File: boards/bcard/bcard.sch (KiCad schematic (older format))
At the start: 13 parts, among them IC1 ATTINY10-TS, P1 BATT, Q1 BC846A

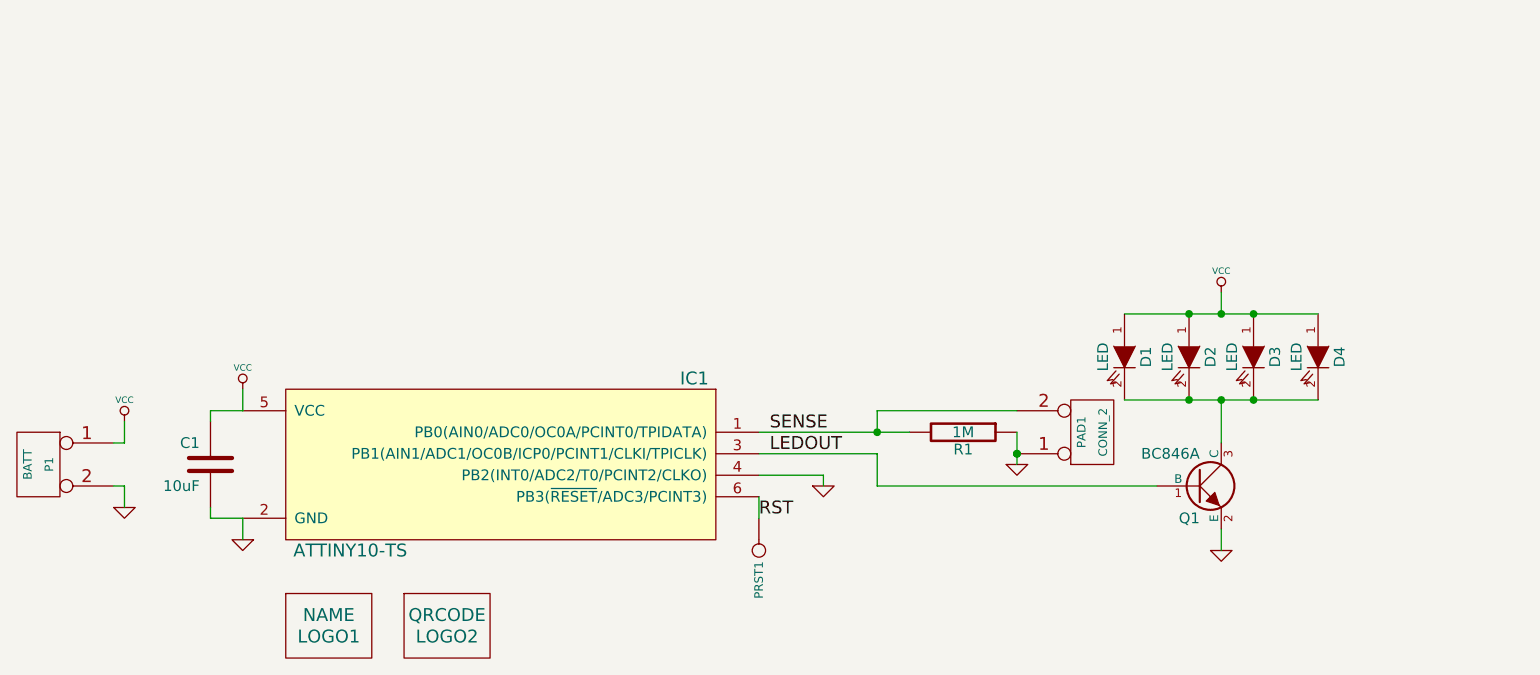
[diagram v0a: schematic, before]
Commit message: first pcb design basically done
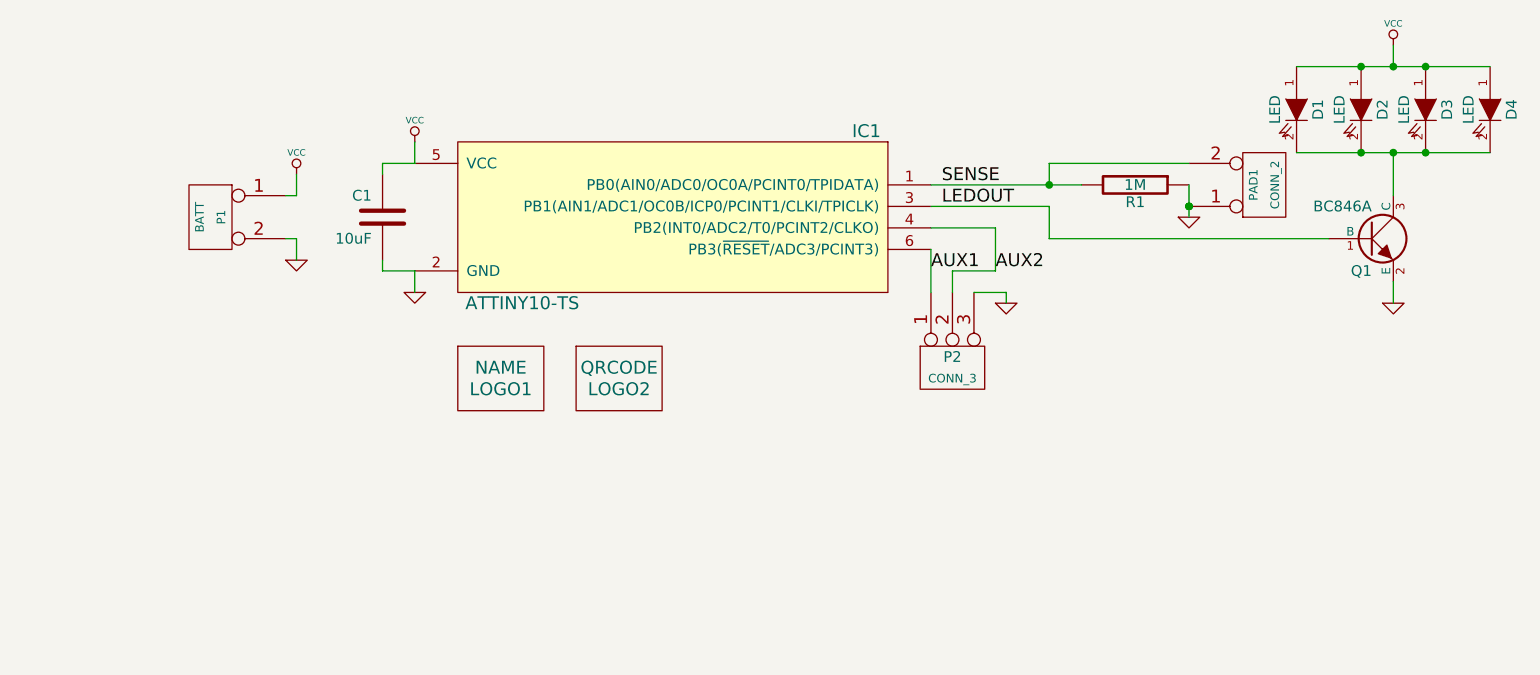
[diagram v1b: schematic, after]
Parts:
- removed PRST1: CONN_1, symbol CONN_1
- added P2: CONN_3, symbol CONN_3
- D1, D2, D3, D4: footprint LED-1206-3D -> SM1206POL
- IC1: footprint DIP-28__300 -> SOT23_6
- LOGO1: footprint (none) -> LOGO
- LOGO2: footprint (none) -> JWCXZ
- PAD1: footprint (none) -> CAPSENSE
- R1: footprint SM0805 -> SM0603
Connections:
- net GND: now also P2.3 (P3); no longer IC1.4 (PB2(INT0/ADC2/T0/PCINT2/CLKO))
- net RST renamed AUX1
- net AUX1: now also P2.1 (P1)
- new net AUX2: IC1.4 (PB2(INT0/ADC2/T0/PCINT2/CLKO)), P2.2 (PM)
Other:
- moved on the sheet: C1, D1, D2, D3, D4, IC1, LOGO1, LOGO2, P1, PAD1, Q1, R1

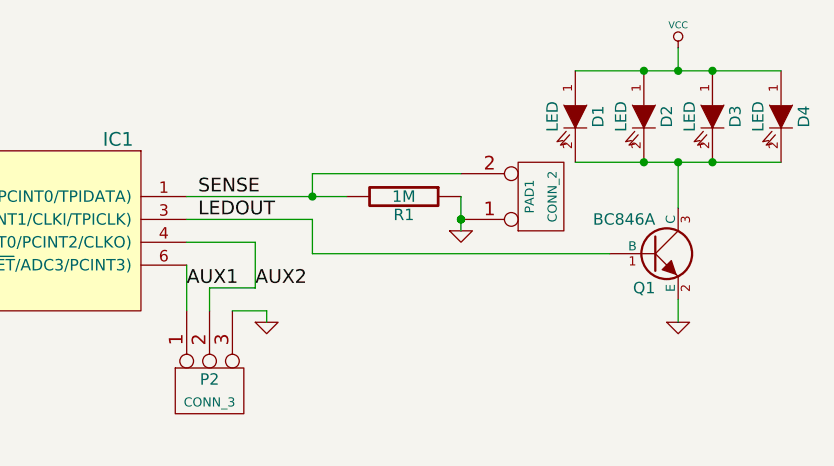
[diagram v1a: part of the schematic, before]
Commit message: almost done with new style
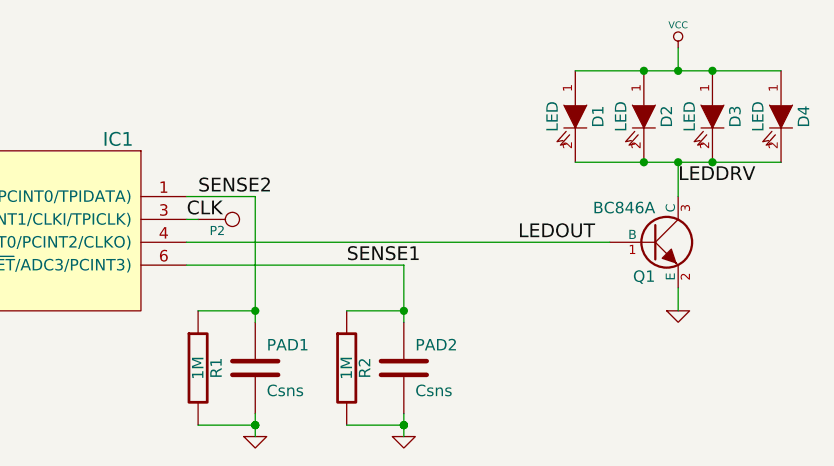
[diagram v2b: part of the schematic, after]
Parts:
- removed P2: CONN_3, symbol CONN_3
- removed PAD1: CONN_2, CAPSENSE, symbol CONN_2
- added P2: CONN_1, PAD, symbol CONN_1
- added PAD1, PAD2: Csns, SIL-2, symbol C
- added R2: 1M, SM0603, symbol R
- D1, D2, D3, D4: footprint SM1206POL -> LED-3mmS
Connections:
- net AUX2 is gone; now on net LEDOUT: IC1.4 (PB2(INT0/ADC2/T0/PCINT2/CLKO))
- net GND: now also R1.2, PAD1.2, PAD2.2, R2.2; no longer R1.1
- net LEDOUT: no longer IC1.3 (PB1(AIN1/ADC1/OC0B/ICP0/PCINT1/CLKI/TPICLK))
- net LEDDRV: now reaches D1.2 (K), D2.2 (K), D3.2 (K), D4.2 (K), Q1.3 (C)
- net AUX1 renamed SENSE1
- net SENSE1: now also PAD2.1, R2.1
- net SENSE renamed SENSE2
- net SENSE2: now also R1.1, PAD1.1; no longer R1.2
- new net CLK: IC1.3 (PB1(AIN1/ADC1/OC0B/ICP0/PCINT1/CLKI/TPICLK)), P2.1
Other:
- moved on the sheet: Q1, R1
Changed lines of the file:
@@
-EESchema Schematic File Version 2  date Thu 29 Mar 2012 05:30:36 PM EDT
+EESchema Schematic File Version 2  date Fri 25 May 2012 11:36:53 AM EDT
 LIBS:power
 LIBS:device
@@
 Sheet 1 1
 Title "bcard"
-Date "29 mar 2012"
+Date "25 may 2012"
 Rev "1.0"
 Comp "J. Colosimo"
@@
 F 0 "D4" H 8600 3150 50  0000 C CNN
 F 1 "LED" H 8600 2950 50  0000 C CNN
-F 2 "SM1206POL" H 8600 3050 50  0001 C CNN
+F 2 "LED-3mmS" H 8600 3050 50  0001 C CNN
 F 4 "APT3216QBC/D" H 8600 3050 60  0001 C CNN "Part"
 F 5 "http://search.digikey.com/us/en/products/APT3216QBC%2FD/754-1439-1-ND/2163797" H 8600 3050 60  0001 C CNN "URL"
@@
 F 0 "D3" H 8300 3150 50  0000 C CNN
 F 1 "LED" H 8300 2950 50  0000 C CNN
-F 2 "SM1206POL" H 8300 3050 50  0001 C CNN
+F 2 "LED-3mmS" H 8300 3050 50  0001 C CNN
 F 4 "APT3216QBC/D" H 8300 3050 60  0001 C CNN "Part"
 F 5 "http://search.digikey.com/us/en/products/APT3216QBC%2FD/754-1439-1-ND/2163797" H 8300 3050 60  0001 C CNN "URL"
@@
 F 0 "D2" H 8000 3150 50  0000 C CNN
 F 1 "LED" H 8000 2950 50  0000 C CNN
-F 2 "SM1206POL" H 8000 3050 50  0001 C CNN
+F 2 "LED-3mmS" H 8000 3050 50  0001 C CNN
 F 4 "APT3216QBC/D" H 8000 3050 60  0001 C CNN "Part"
 F 5 "http://search.digikey.com/us/en/products/APT3216QBC%2FD/754-1439-1-ND/2163797" H 8000 3050 60  0001 C CNN "URL"
@@
 L R R1
 U 1 1 4F57ACF5
-P 6950 3400
-F 0 "R1" V 7030 3400 50  0000 C CNN
-F 1 "1M" V 6950 3400 50  0000 C CNN
-F 2 "SM0603" V 7050 3400 50  0001 C CNN
-F 4 "RC0603JR-071ML" V 6950 3400 60  0001 C CNN "Part"
-F 5 "http://search.digikey.com/us/en/products/RC0603JR-071ML/311-1.0MGRCT-ND/729625" V 6950 3400 60  0001 C CNN "URL"
-	1    6950 3400
-	0    1    1    0
+P 6050 4150
+F 0 "R1" V 6130 4150 50  0000 C CNN
+F 1 "1M" V 6050 4150 50  0000 C CNN
+F 2 "SM0603" V 6150 4150 50  0001 C CNN
+F 4 "RC0603JR-071ML" V 6050 4150 60  0001 C CNN "Part"
+F 5 "http://search.digikey.com/us/en/products/RC0603JR-071ML/311-1.0MGRCT-ND/729625" V 6050 4150 60  0001 C CNN "URL"
+	1    6050 4150
+	1    0    0    -1
 $EndComp
 $Comp
@@
 L GND #PWR03
 U 1 1 4F57A9AD
-P 8150 3950
-F 0 "#PWR03" H 8150 3950 30  0001 C CNN
-F 1 "GND" H 8150 3880 30  0001 C CNN
-	1    8150 3950
+P 8150 3900
+F 0 "#PWR03" H 8150 3900 30  0001 C CNN
+F 1 "GND" H 8150 3830 30  0001 C CNN
+	1    8150 3900
 	1    0    0    -1
 $EndComp
@@
 F 0 "D1" H 7700 3150 50  0000 C CNN
 F 1 "LED" H 7700 2950 50  0000 C CNN
-F 2 "SM1206POL" H 7700 3050 50  0001 C CNN
+F 2 "LED-3mmS" H 7700 3050 50  0001 C CNN
 F 4 "APT3216QBC/D" H 7700 3050 60  0001 C CNN "Part"
 F 5 "http://search.digikey.com/us/en/products/APT3216QBC%2FD/754-1439-1-ND/2163797" H 7700 3050 60  0001 C CNN "URL"
@@
 L BC846A Q1
 U 1 1 4F57A871
-P 8050 3650
-F 0 "Q1" H 8050 3500 50  0000 R CNN
-F 1 "BC846A" H 8050 3800 50  0000 R CNN
-F 2 "SOT323" H 8050 3900 50  0001 C CNN
-F 4 "BC846A" H 8050 3650 60  0001 C CNN "Part"
-F 5 "http://search.digikey.com/us/en/products/BC846A,215/568-4866-1-ND/2122195" H 8050 3650 60  0001 C CNN "URL"
-	1    8050 3650
+P 8050 3600
+F 0 "Q1" H 8050 3450 50  0000 R CNN
+F 1 "BC846A" H 8050 3750 50  0000 R CNN
+F 2 "SOT323" H 8050 3850 50  0001 C CNN
+F 4 "BC846A" H 8050 3600 60  0001 C CNN "Part"
+F 5 "http://search.digikey.com/us/en/products/BC846A,215/568-4866-1-ND/2122195" H 8050 3600 60  0001 C CNN "URL"
+	1    8050 3600
 	1    0    0    -1
 $EndComp
@@
 $EndComp
 $Comp
-L GND #PWR07
-U 1 1 4F72D7B3
-P 7200 3550
-F 0 "#PWR07" H 7200 3550 30  0001 C CNN
-F 1 "GND" H 7200 3480 30  0001 C CNN
-	1    7200 3550
-	1    0    0    -1
-$EndComp
-$Comp
 L LOGO LOGO1
 U 1 1 4F737976
@@
 	1    0    0    -1
 $EndComp
+Text Label 6050 3400 0    60   ~ 0
+SENSE2
+Text Label 7450 3600 0    60   ~ 0
+LEDOUT
 $Comp
 L LOGO LOGO2
@@
 	1    0    0    -1
 $EndComp
-Text Label 6050 3400 0    60   ~ 0
-SENSE
-Text Label 6050 3500 0    60   ~ 0
-LEDOUT
-Text Label 6000 3800 0    60   ~ 0
-AUX1
-$Comp
-L CONN_2 PAD1
-U 1 1 4F740194
-P 7550 3400
-F 0 "PAD1" V 7500 3400 40  0000 C CNN
-F 1 "CONN_2" V 7600 3400 40  0000 C CNN
-F 2 "CAPSENSE" V 7700 3400 40  0001 C CNN
-	1    7550 3400
-	1    0    0    1
-$EndComp
-Text Label 6300 3800 0    60   ~ 0
-AUX2
-$Comp
-L CONN_3 P2
-U 1 1 4F74D36B
-P 6100 4250
-F 0 "P2" V 6050 4250 50  0000 C CNN
-F 1 "CONN_3" V 6150 4250 40  0000 C CNN
-	1    6100 4250
-	0    -1   1    0
+Text Label 8150 3350 0    60   ~ 0
+LEDDRV
+$Comp
+L C PAD1
+U 1 1 4FBF9DE9
+P 6300 4150
+F 0 "PAD1" H 6350 4250 50  0000 L CNN
+F 1 "Csns" H 6350 4050 50  0000 L CNN
+F 2 "SIL-2" H 6350 4150 50  0001 C CNN
+	1    6300 4150
+	1    0    0    -1
+$EndComp
+$Comp
+L GND #PWR07
+U 1 1 4FBF9E84
+P 6300 4450
+F 0 "#PWR07" H 6300 4450 30  0001 C CNN
+F 1 "GND" H 6300 4380 30  0001 C CNN
+	1    6300 4450
+	1    0    0    -1
+$EndComp
+$Comp
+L R R2
+U 1 1 4FBF9F06
+P 6700 4150
+F 0 "R2" V 6780 4150 50  0000 C CNN
+F 1 "1M" V 6700 4150 50  0000 C CNN
+F 2 "SM0603" V 6800 4150 50  0001 C CNN
+F 4 "RC0603JR-071ML" V 6700 4150 60  0001 C CNN "Part"
+F 5 "http://search.digikey.com/us/en/products/RC0603JR-071ML/311-1.0MGRCT-ND/729625" V 6700 4150 60  0001 C CNN "URL"
+	1    6700 4150
+	1    0    0    -1
+$EndComp
+$Comp
+L C PAD2
+U 1 1 4FBF9F0C
+P 6950 4150
+F 0 "PAD2" H 7000 4250 50  0000 L CNN
+F 1 "Csns" H 7000 4050 50  0000 L CNN
+F 2 "SIL-2" H 7000 4150 50  0001 C CNN
+	1    6950 4150
+	1    0    0    -1
 $EndComp
 $Comp
 L GND #PWR08
-U 1 1 4F74D45B
-P 6350 3950
-F 0 "#PWR08" H 6350 3950 30  0001 C CNN
-F 1 "GND" H 6350 3880 30  0001 C CNN
-	1    6350 3950
+U 1 1 4FBF9F12
+P 6950 4450
+F 0 "#PWR08" H 6950 4450 30  0001 C CNN
+F 1 "GND" H 6950 4380 30  0001 C CNN
+	1    6950 4450
+	1    0    0    -1
+$EndComp
+Text Label 6700 3700 0    60   ~ 0
+SENSE1
+$Comp
+L CONN_1 P2
+U 1 1 4FBFA0FD
+P 6200 3500
+F 0 "P2" H 6100 3450 40  0000 L CNN
+F 1 "CONN_1" H 6200 3555 30  0001 C CNN
+F 2 "PAD" H 6200 3655 30  0001 C CNN
+	1    6200 3500
 	1    0    0    -1
 $EndComp
@@
 Connection ~ 8300 2850
 Wire Wire Line
-	8150 3250 8150 3450
+	8150 3250 8150 3400
 Connection ~ 8150 3250
 Wire Wire Line
-	8150 3850 8150 3950
+	8150 3800 8150 3900
 Wire Wire Line
 	3000 3650 3050 3650
@@
 	3050 3650 3050 3750
 Wire Wire Line
-	6000 3400 6700 3400
-Wire Wire Line
-	7200 3300 6550 3300
-Wire Wire Line
-	6550 3300 6550 3400
-Connection ~ 6550 3400
-Wire Wire Line
-	6000 3500 6550 3500
-Wire Wire Line
-	6550 3500 6550 3650
-Wire Wire Line
-	6550 3650 7850 3650
-Wire Wire Line
-	7200 3550 7200 3400
-Connection ~ 7200 3500
-Connection ~ 7200 3500
-Wire Wire Line
-	6000 3700 6000 3900
-Wire Wire Line
-	6000 3600 6300 3600
-Wire Wire Line
-	6300 3600 6300 3800
-Wire Wire Line
-	6300 3800 6100 3800
-Wire Wire Line
-	6100 3800 6100 3900
-Wire Wire Line
-	6350 3950 6350 3900
-Wire Wire Line
-	6350 3900 6200 3900
+	6000 3600 7850 3600
+Wire Wire Line
+	6050 3900 6300 3900
+Wire Wire Line
+	6300 3950 6300 3400
+Wire Wire Line
+	6300 4350 6300 4450
+Wire Wire Line
+	6300 4400 6050 4400
+Connection ~ 6300 4400
+Connection ~ 6300 4400
+Wire Wire Line
+	6700 3900 6950 3900
+Wire Wire Line
+	6950 3950 6950 3700
+Wire Wire Line
+	6950 4350 6950 4450
+Wire Wire Line
+	6950 4400 6700 4400
+Connection ~ 6950 4400
+Connection ~ 6950 4400
+Wire Wire Line
+	6300 3400 6000 3400
+Connection ~ 6300 3900
+Wire Wire Line
+	6950 3700 6000 3700
+Connection ~ 6950 3900
+Wire Wire Line
+	6000 3500 6050 3500
+Text Label 6000 3500 0    60   ~ 0
+CLK
 $EndSCHEMATC

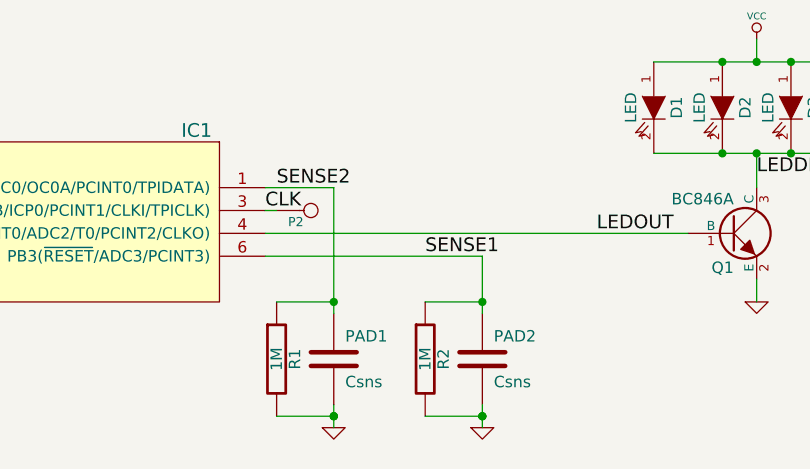
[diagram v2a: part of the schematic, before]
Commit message: finished next revision of bcard -- ready to etch
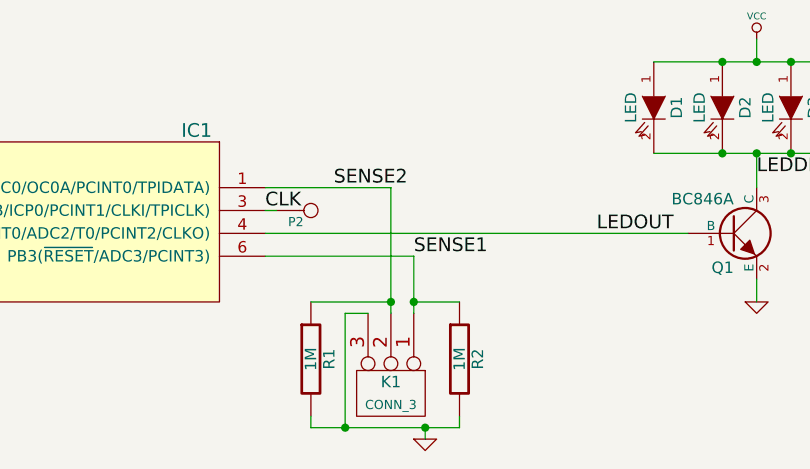
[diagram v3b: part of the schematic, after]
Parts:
- removed PAD1, PAD2: Csns, SIL-2, symbol C
- added K1: CONN_3, SENSOR2, symbol CONN_3
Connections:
- net GND: now also K1.3 (P3)
- net SENSE1: now also K1.1 (P1)
- net SENSE2: now also K1.2 (PM)
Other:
- moved on the sheet: R1, R2
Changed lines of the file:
@@
-EESchema Schematic File Version 2  date Fri 25 May 2012 11:36:53 AM EDT
+EESchema Schematic File Version 2  date Mon 28 May 2012 02:41:33 PM EDT
 LIBS:power
 LIBS:device
@@
 Sheet 1 1
 Title "bcard"
-Date "25 may 2012"
+Date "28 may 2012"
 Rev "1.0"
 Comp "J. Colosimo"
@@
 L R R1
 U 1 1 4F57ACF5
-P 6050 4150
-F 0 "R1" V 6130 4150 50  0000 C CNN
-F 1 "1M" V 6050 4150 50  0000 C CNN
-F 2 "SM0603" V 6150 4150 50  0001 C CNN
-F 4 "RC0603JR-071ML" V 6050 4150 60  0001 C CNN "Part"
-F 5 "http://search.digikey.com/us/en/products/RC0603JR-071ML/311-1.0MGRCT-ND/729625" V 6050 4150 60  0001 C CNN "URL"
-	1    6050 4150
+P 6200 4150
+F 0 "R1" V 6280 4150 50  0000 C CNN
+F 1 "1M" V 6200 4150 50  0000 C CNN
+F 2 "SM0603" V 6300 4150 50  0001 C CNN
+F 4 "RC0603JR-071ML" V 6200 4150 60  0001 C CNN "Part"
+F 5 "http://search.digikey.com/us/en/products/RC0603JR-071ML/311-1.0MGRCT-ND/729625" V 6200 4150 60  0001 C CNN "URL"
+	1    6200 4150
 	1    0    0    -1
 $EndComp
@@
 	1    0    0    -1
 $EndComp
-Text Label 6050 3400 0    60   ~ 0
+Text Label 6300 3400 0    60   ~ 0
 SENSE2
 Text Label 7450 3600 0    60   ~ 0
@@
 LEDDRV
 $Comp
-L C PAD1
-U 1 1 4FBF9DE9
-P 6300 4150
-F 0 "PAD1" H 6350 4250 50  0000 L CNN
-F 1 "Csns" H 6350 4050 50  0000 L CNN
-F 2 "SIL-2" H 6350 4150 50  0001 C CNN
-	1    6300 4150
-	1    0    0    -1
-$EndComp
-$Comp
-L GND #PWR07
-U 1 1 4FBF9E84
-P 6300 4450
-F 0 "#PWR07" H 6300 4450 30  0001 C CNN
-F 1 "GND" H 6300 4380 30  0001 C CNN
-	1    6300 4450
-	1    0    0    -1
-$EndComp
-$Comp
 L R R2
 U 1 1 4FBF9F06
-P 6700 4150
-F 0 "R2" V 6780 4150 50  0000 C CNN
-F 1 "1M" V 6700 4150 50  0000 C CNN
-F 2 "SM0603" V 6800 4150 50  0001 C CNN
-F 4 "RC0603JR-071ML" V 6700 4150 60  0001 C CNN "Part"
-F 5 "http://search.digikey.com/us/en/products/RC0603JR-071ML/311-1.0MGRCT-ND/729625" V 6700 4150 60  0001 C CNN "URL"
-	1    6700 4150
-	1    0    0    -1
-$EndComp
-$Comp
-L C PAD2
-U 1 1 4FBF9F0C
-P 6950 4150
-F 0 "PAD2" H 7000 4250 50  0000 L CNN
-F 1 "Csns" H 7000 4050 50  0000 L CNN
-F 2 "SIL-2" H 7000 4150 50  0001 C CNN
-	1    6950 4150
-	1    0    0    -1
-$EndComp
-$Comp
-L GND #PWR08
-U 1 1 4FBF9F12
-P 6950 4450
-F 0 "#PWR08" H 6950 4450 30  0001 C CNN
-F 1 "GND" H 6950 4380 30  0001 C CNN
-	1    6950 4450
-	1    0    0    -1
-$EndComp
-Text Label 6700 3700 0    60   ~ 0
+P 6850 4150
+F 0 "R2" V 6930 4150 50  0000 C CNN
+F 1 "1M" V 6850 4150 50  0000 C CNN
+F 2 "SM0603" V 6950 4150 50  0001 C CNN
+F 4 "RC0603JR-071ML" V 6850 4150 60  0001 C CNN "Part"
+F 5 "http://search.digikey.com/us/en/products/RC0603JR-071ML/311-1.0MGRCT-ND/729625" V 6850 4150 60  0001 C CNN "URL"
+	1    6850 4150
+	1    0    0    -1
+$EndComp
+Text Label 6650 3700 0    60   ~ 0
 SENSE1
 $Comp
@@
 	1    0    0    -1
 $EndComp
+Text Label 6000 3500 0    60   ~ 0
+CLK
+$Comp
+L CONN_3 K1
+U 1 1 4FC3BBC8
+P 6550 4300
+F 0 "K1" V 6500 4300 50  0000 C CNN
+F 1 "CONN_3" V 6600 4300 40  0000 C CNN
+F 2 "SENSOR2" V 6700 4300 40  0001 C CNN
+	1    6550 4300
+	0    1    1    0
+$EndComp
+$Comp
+L GND #PWR07
+U 1 1 4FC3BCB2
+P 6700 4500
+F 0 "#PWR07" H 6700 4500 30  0001 C CNN
+F 1 "GND" H 6700 4430 30  0001 C CNN
+	1    6700 4500
+	1    0    0    -1
+$EndComp
 Wire Wire Line
 	3050 3350 3050 3450
@@
 	6000 3600 7850 3600
 Wire Wire Line
-	6050 3900 6300 3900
-Wire Wire Line
-	6300 3950 6300 3400
-Wire Wire Line
-	6300 4350 6300 4450
-Wire Wire Line
-	6300 4400 6050 4400
-Connection ~ 6300 4400
-Connection ~ 6300 4400
-Wire Wire Line
-	6700 3900 6950 3900
-Wire Wire Line
-	6950 3950 6950 3700
-Wire Wire Line
-	6950 4350 6950 4450
-Wire Wire Line
-	6950 4400 6700 4400
-Connection ~ 6950 4400
-Connection ~ 6950 4400
-Wire Wire Line
-	6300 3400 6000 3400
-Connection ~ 6300 3900
-Wire Wire Line
-	6950 3700 6000 3700
-Connection ~ 6950 3900
+	6200 3900 6550 3900
+Wire Wire Line
+	6550 3950 6550 3400
+Wire Wire Line
+	6850 3900 6650 3900
+Wire Wire Line
+	6650 3950 6650 3700
+Wire Wire Line
+	6550 3400 6000 3400
+Connection ~ 6550 3900
+Wire Wire Line
+	6650 3700 6000 3700
+Connection ~ 6650 3900
 Wire Wire Line
 	6000 3500 6050 3500
-Text Label 6000 3500 0    60   ~ 0
-CLK
+Wire Wire Line
+	6850 4450 6850 4400
+Wire Wire Line
+	6850 4450 6200 4450
+Wire Wire Line
+	6700 4450 6700 4500
+Wire Wire Line
+	6200 4450 6200 4400
+Connection ~ 6700 4450
+Wire Wire Line
+	6450 3950 6350 3950
+Wire Wire Line
+	6350 3950 6350 4450
+Connection ~ 6350 4450
 $EndSCHEMATC
